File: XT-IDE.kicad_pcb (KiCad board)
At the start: 2 copper layers, 105.7 x 96 mm, 51 parts, among them J1 Power output, J2 Conn_01x02, J3 External LED, J4 Conn_01x02, J5 Conn_02x05_Odd_Even, P6 CONN_1, P7 CONN_1, SW1 DIPS_06, SW2 DIPS_04, SW3 DPDT, SW4 DPDT, SW5 SPDT, SW6 SPDT, U1 74HCT573, U10 74HCT688, U11 74HCT245, U12 74LS33, U2 74HCT573, U3 74HCT245, U4 74HCT04, U5 74HCT32, U6 74HCT04, U7 74HCT138, U8 74HCT688, U9 28C256

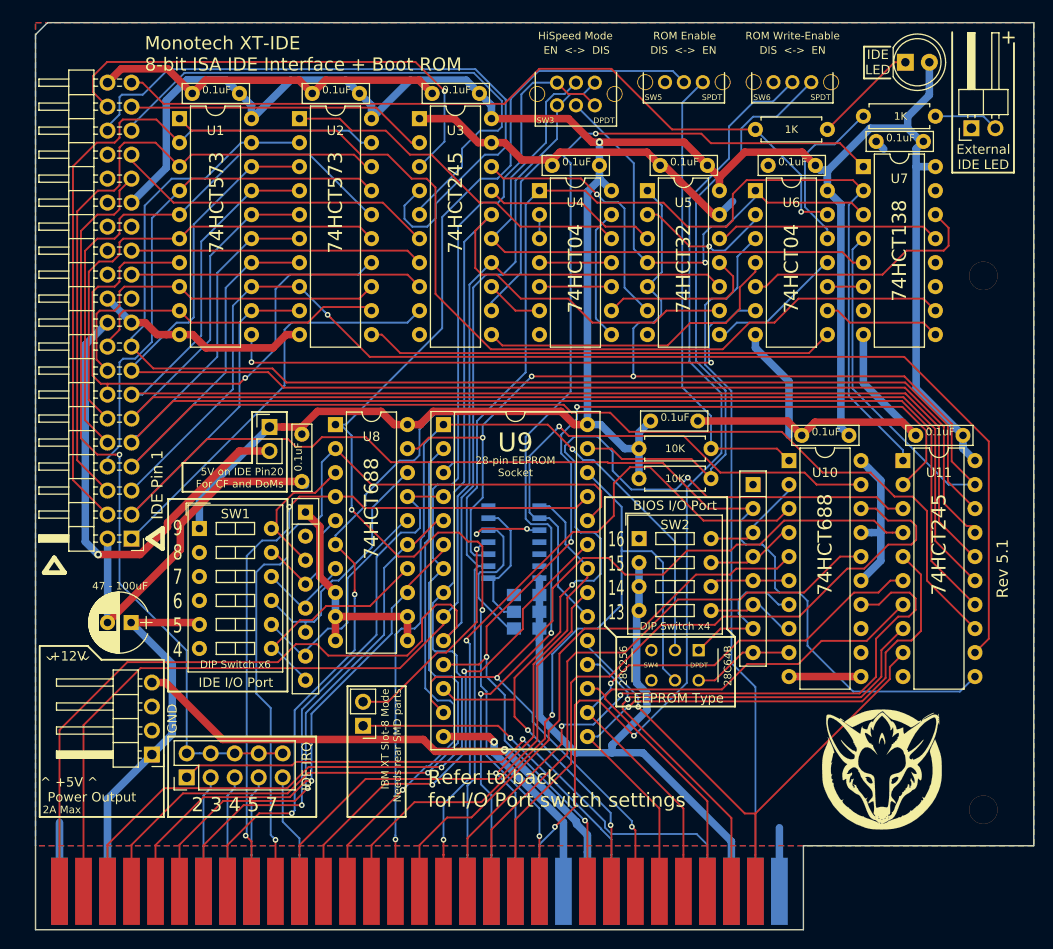
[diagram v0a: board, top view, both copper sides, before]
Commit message: Add files via upload
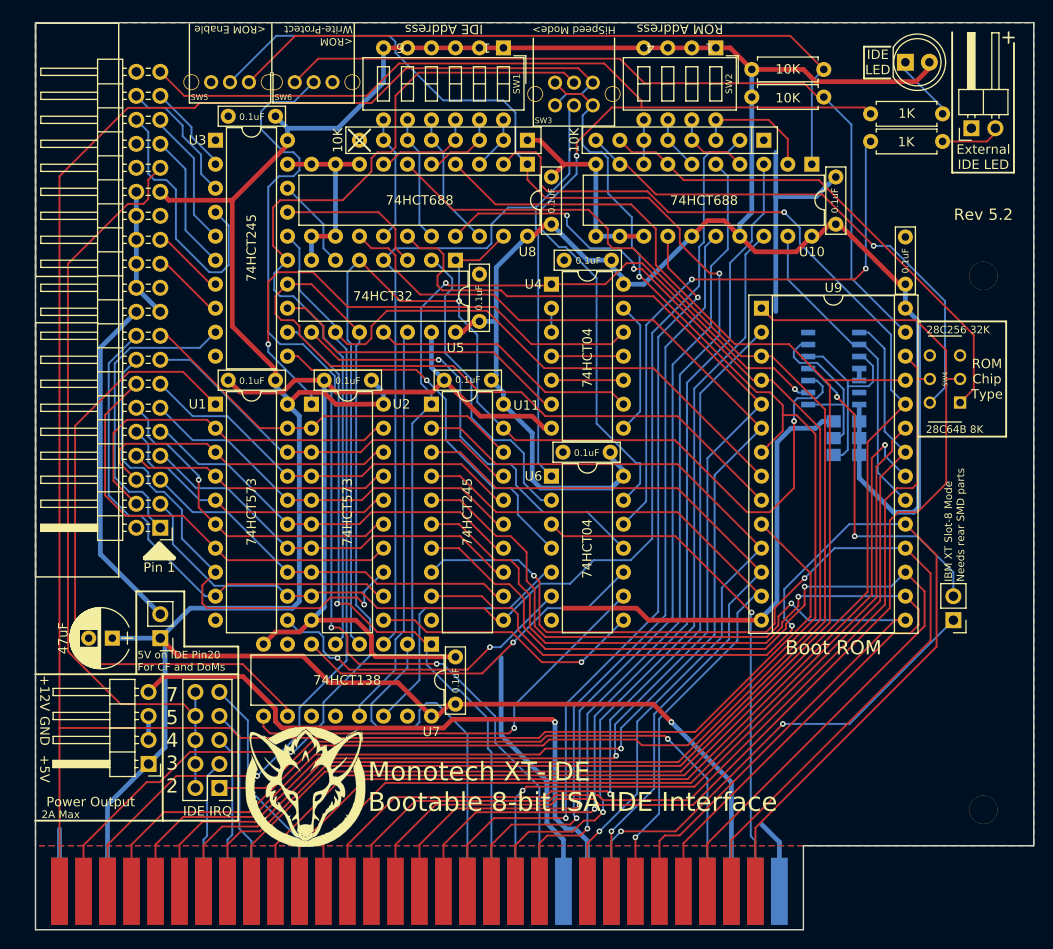
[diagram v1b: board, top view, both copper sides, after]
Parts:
- C1, C10, C11, C13, C2, C3, C4, C5, C6, C7, C8, C9: value C -> 0.1uF
- IDE1: footprint Custom:Pin_Header_Angled_2x20_ShortSilkS -> Custom:Pin_Header_Angled_2x20_Pitch2.54mm_Shrouded
- RP1, RP2: value 10k -> 10K
- SW1: value DIPS_06 -> IDE Address; footprint Buttons_Switches_THT:SW_DIP_x6_W7.62mm_Slide -> Buttons_Switches_THT:SW_DIP_x6_W7.62mm_Slide_LowProfile
- SW2: value DIPS_04 -> ROM Address; footprint Buttons_Switches_THT:SW_DIP_x4_W7.62mm_Slide -> Buttons_Switches_THT:SW_DIP_x4_W7.62mm_Slide_LowProfile
- U9: value 28C256 -> 28C64B/28C256
- moved REF*** 82.5 mm to (204.6, 117.0)
- moved U7 68.2 mm to (147.3, 131.8), turned to 270 degrees
- moved J2 63.5 mm to (202.6, 129.3)
- moved G*** 61.1 mm to (134.0, 146.9)
- moved C8 60.7 mm to (190.1, 87.4), turned to 90 degrees
- moved SW1 60.2 mm to (154.9, 68.7), turned to 270 degrees
- moved SW2 52.6 mm to (177.4, 68.7), turned to 270 degrees
- moved SW6 50.7 mm to (134.8, 72.3)
- moved C10 50.4 mm to (149.9, 138.2), turned to 90 degrees
- moved U11 50.3 mm to (147.3, 106.4)
- moved SW5 48.0 mm to (126.0, 72.3)
- moved RP1 45.8 mm to (157.5, 78.5), turned to 180 degrees
- moved R3 42.1 mm to (181.2, 73.9)
- moved R4 41.9 mm to (181.2, 71.0)
- moved SW4 41.7 mm to (201.7, 103.8), turned to 180 degrees
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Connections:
- RP1 pad 2: (no net) -> Net-(RP1-Pad2)
- RP1 pad 8: Net-(RP1-Pad8) -> (no net)
- SW1 pad 10: Net-(RP1-Pad5) -> Net-(RP1-Pad4)
- SW1 pad 11: Net-(RP1-Pad4) -> Net-(RP1-Pad3)
- SW1 pad 12: Net-(RP1-Pad3) -> Net-(RP1-Pad2)
- SW1 pad 7: Net-(RP1-Pad8) -> Net-(RP1-Pad7)
- SW1 pad 8: Net-(RP1-Pad7) -> Net-(RP1-Pad6)
- SW1 pad 9: Net-(RP1-Pad6) -> Net-(RP1-Pad5)
- SW6 pad 1: ROM_WE -> (no net)
- SW6 pad 3: (no net) -> ROM_WE
- U8 pad 14: Net-(RP1-Pad8) -> Net-(RP1-Pad7)
- U8 pad 16: Net-(RP1-Pad7) -> Net-(RP1-Pad6)
- U8 pad 18: Net-(RP1-Pad6) -> Net-(RP1-Pad5)
- U8 pad 3: Net-(RP1-Pad3) -> Net-(RP1-Pad2)
- U8 pad 5: Net-(RP1-Pad4) -> Net-(RP1-Pad3)
- U8 pad 7: Net-(RP1-Pad5) -> Net-(RP1-Pad4)
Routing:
- net A0: track 138.7 -> 239.7 mm
- net D4: track 140.8 -> 42.5 mm
- net D5: track 138.5 -> 42.5 mm
- net A4: track 55.0 -> 150.3 mm
- net D3: track 137.8 -> 42.5 mm
- net D6: track 134.9 -> 41.4 mm, vias 1 -> 0
- net D2: track 135.5 -> 42.5 mm
- net D0: track 134.5 -> 42.5 mm
- net D1: track 134.5 -> 42.5 mm
- net A5: track 56.2 -> 146.4 mm
- net A6: track 60.1 -> 150.3 mm, vias 1 -> 2
- net A8: track 76.8 -> 161.1 mm, vias 2 -> 0
- net A7: track 73.0 -> 156.3 mm, vias 2 -> 0
- net A9: track 86.8 -> 160.4 mm
- net IOW: track 141.3 -> 73.0 mm, vias 3 -> 1
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- added copper zone on F.Cu, net GND
- removed copper zone on F.Cu, net VCC
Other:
- outline, holes or cut-outs redrawn
- net class Power: trace_width 0.8 -> 0.5; via_dia 0.8 -> 0.6; via_drill 0.4 -> 0.3
- board text added: "1 000011111111 2 111100001111 3 001100110011 4 010101010101"
- board text added: "1 0011111111111111111111111111111111 2 1100000000000000001111111111111111 3 0100000000111111110000000011111111 4 1100001111000011110000111100001111 5 1100110011001100110011001100110011 6 1101010101010101010101010101010101"
- board text added: "1 2 3 4"
- board text added: "1 2 3 4 5 6"
- board text added: "1 4"
- board text added: "1 6"
- board text added: "28C256 32K"
- board text added: "28C64B 8K"
- board text added: "7 5 4 3 2"
- board text added: "<ROM Enable"
- board text added: "<ROM Write-Protect"
- board text added: "=32KiB ROM Support"
- board text added: "Boot ROM"
- board text added: "Enable the ROM Write-Protect once system is up and running the way intended, to prevent accidental re-flashing."
- board text added: "HiSpeed Mode>"
- board text added: "IDE Address"
- board text added: "IDE Address Switch Settings"
- board text added: "Monotech XT-IDE Bootable 8-bit ISA IDE Interface"
- board text added: "ROM Address"
- board text added: "ROM Address Switch Settings"
- board text added: "ROM Chip Type"
- board text added: "Rev 5.2"
- board text removed: "0.1uF"
- board text removed: "10K"
- board text removed: "16 000011111111 15 111100001111 14 001100110011 13 010101010101"
- board text removed: "16 15 14 13"
- board text removed: "1K"
- board text removed: "2 3 4 5 7"
- board text removed: "28-pin EEPROM Socket"
- board text removed: "28C256"
- board text removed: "28C64B"
- board text removed: "47 - 100uF"
- board text removed: "74HCT04"
- board text removed: "74HCT138"
- board text removed: "74HCT245"
- board text removed: "74HCT32"
- board text removed: "74HCT573"
- board text removed: "74HCT688"
- board text removed: "74LS33"
- board text removed: "9 0011111111111111111111111111111111 8 1100000000000000001111111111111111 7 0100000000111111110000000011111111 6 1100001111000011110000111100001111 5 1100110011001100110011001100110011 4 1101010101010101010101010101010101"
- board text removed: "9 8 7 6 5 4"
- board text removed: "=32KB ROM Support"
- board text removed: "BIOS I/O Port"
- board text removed: "Boot ROM Enable"
- board text removed: "Boot ROM I/O Address Switch Settings"
- board text removed: "Boot ROM Write Enable"
- board text removed: "DIP Switch x4"
- board text removed: "DIP Switch x6"
- board text removed: "DIS <-> EN"
- board text removed: "Disable the "write-enable" once system is up and running the way intended, to prevent accidental re-flashing."
- board text removed: "EEPROM Type"
- board text removed: "EN <-> DIS"
- board text removed: "HiSpeed Mode"
- board text removed: "IDE I/O Address Switch Settings"
- board text removed: "IDE I/O Port"
- board text removed: "IDE Pin 1"
- board text removed: "Monotech XT-IDE 8-bit ISA IDE Interface + Boot ROM"
- board text removed: "ROM Enable"
- board text removed: "ROM Write-Enable"
- board text removed: "Refer to back for I/O Port switch settings"
- board text removed: "Rev 5.1"
- board text removed: "^ +5V ^"
- board text removed: "^ ^"
